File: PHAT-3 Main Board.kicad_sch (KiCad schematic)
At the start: 20 parts, among them P1 Power Terminal Block, P2 Power Terminal Block, P3 Power Terminal Block, P4 Power Terminal Block, Q1 IRLZ44N, U1 AHT21, U10 Logic Level Converter, U2 ESP32-S3 Dual-core SX1262, U3 BME280, U4 GY-521 MPU-6050, U5 LM2596, U6 GT-7U, U7 SCD41, U8 uCAM-III, U9 SD Card Reader

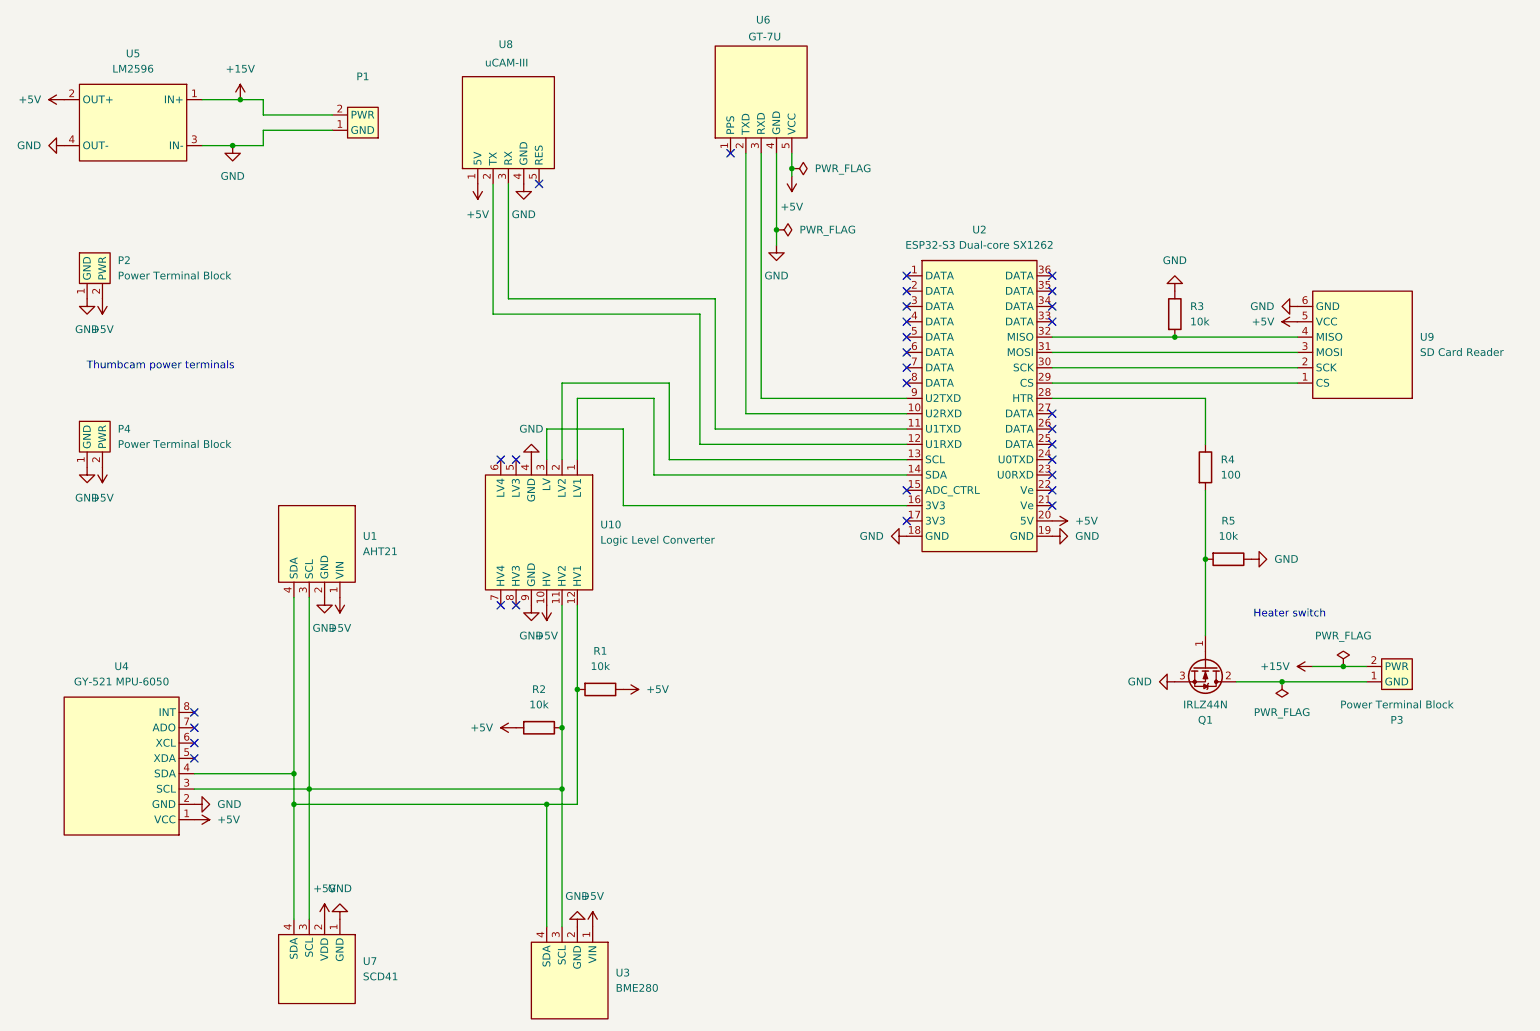
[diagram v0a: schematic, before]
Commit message: Rewired Everything Again
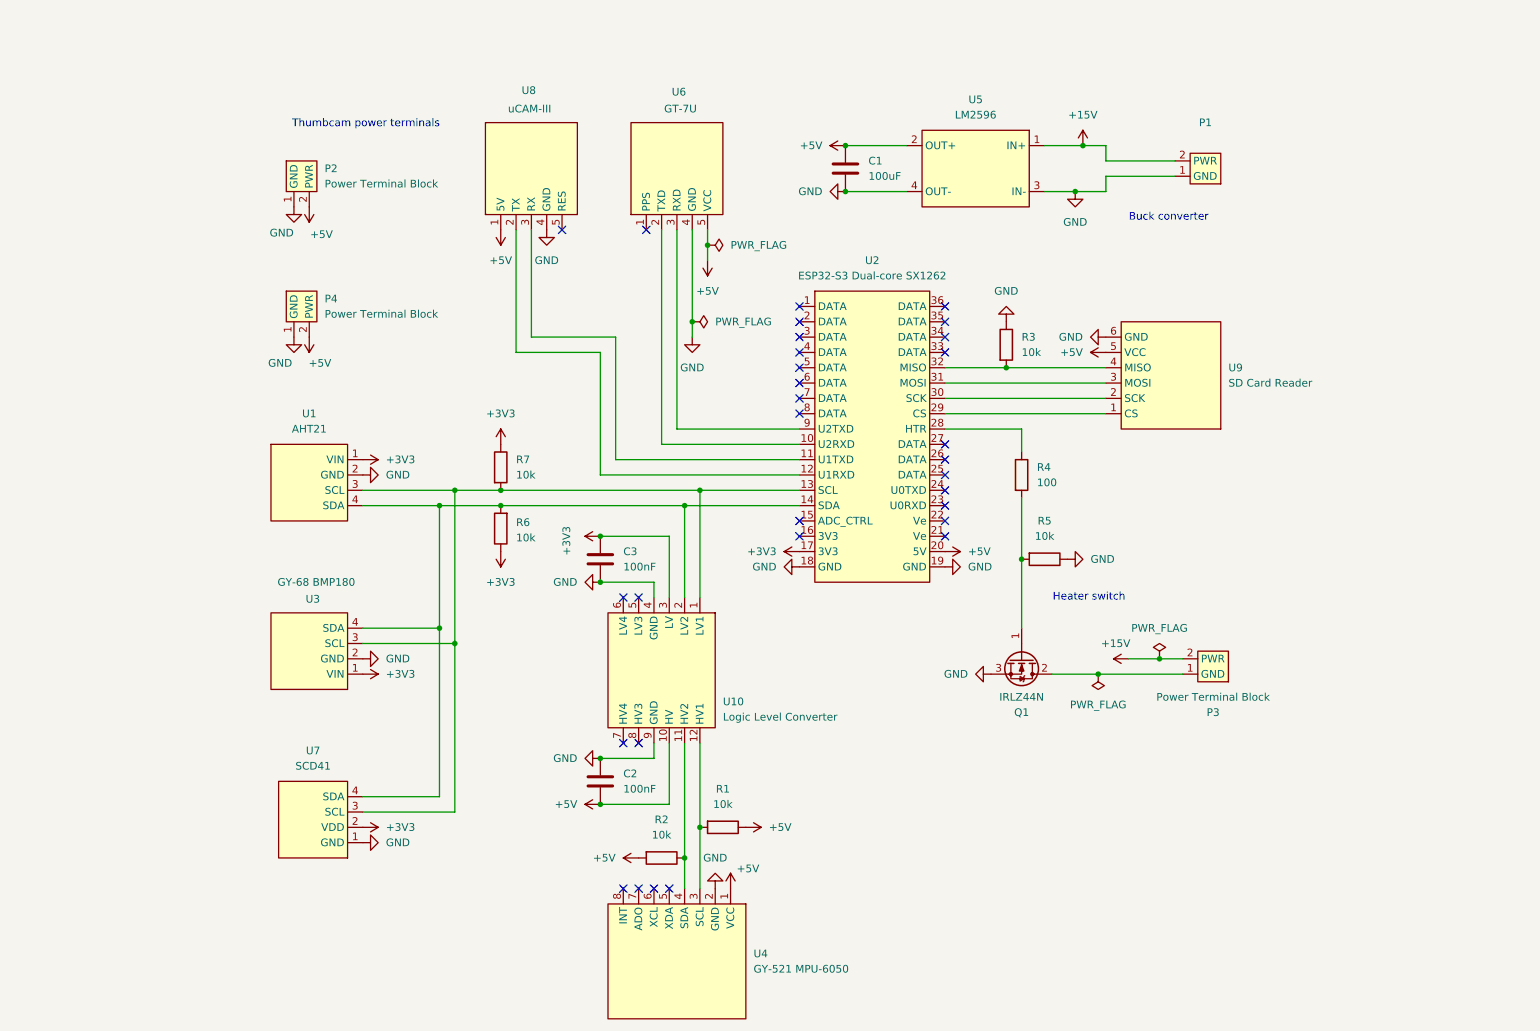
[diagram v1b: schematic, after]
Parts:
- removed U3: BME280, Actual Footprint Library:BME280, symbol Footprint Library:BME280
- added C1: 100uF, Capacitor_THT:C_Radial_D5.0mm_H11.0mm_P2.00mm, symbol Device:C
- added C2, C3: 100nF, Capacitor_THT:C_Disc_D3.0mm_W2.0mm_P2.50mm, symbol Device:C
- added R6, R7: 10k, Resistor_THT:R_Axial_DIN0207_L6.3mm_D2.5mm_P10.16mm_Horizontal, symbol Device:R
- added U3: GY-68 BMP180, Actual Footprint Library:GY-68 BMP180, symbol Footprint Library:GY-68 BMP180
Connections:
- net +5V: now also C1.1, C2.2; no longer U1.1 (VIN), U7.2 (VDD)
- net GND: now also C1.2, C2.1, C3.2, U3.2 (GND)
- net at U2.13 (SCL): now also U1.3 (SCL), U10.1 (LV1), U7.3 (SCL), R7.2, U3.3 (SCL); no longer U10.2 (LV2)
- net at U2.14 (SDA): now also U1.4 (SDA), U10.2 (LV2), U7.4 (SDA), R6.2, U3.4 (SDA); no longer U10.1 (LV1)
- net at U2.16 (3V3): no longer U10.3 (LV)
- net +3V3: now reaches U2.17 (3V3)
- net +3V3: now also U1.1 (VIN), U10.3 (LV), U7.2 (VDD), C3.1, R6.1, R7.1, U3.1 (VIN)
- new net: R2.1, U10.11 (HV2), U4.4 (SDA)
- new net: R1.2, U10.12 (HV1), U4.3 (SCL)
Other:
- note added: "Buck converter"
- moved on the sheet: P1, P2, P3, P4, Q1, R1, R2, R3, R4, R5, U10, U2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
